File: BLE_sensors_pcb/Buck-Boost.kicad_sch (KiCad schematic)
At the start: 6 parts, among them U3 TPS63031DSK

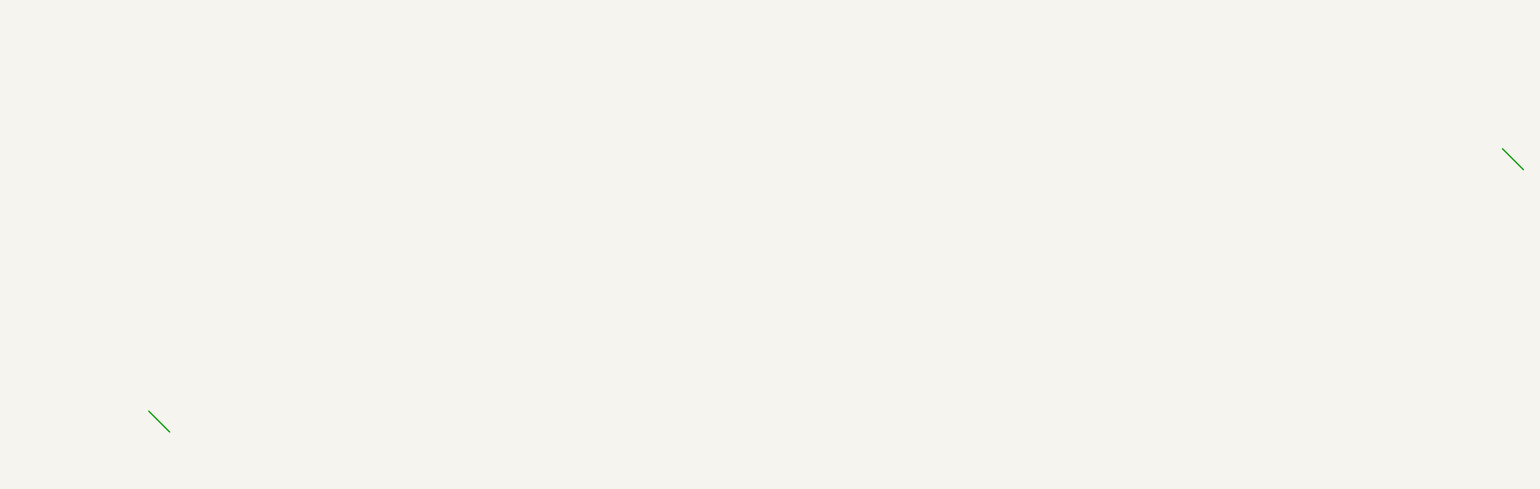
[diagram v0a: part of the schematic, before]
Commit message: save
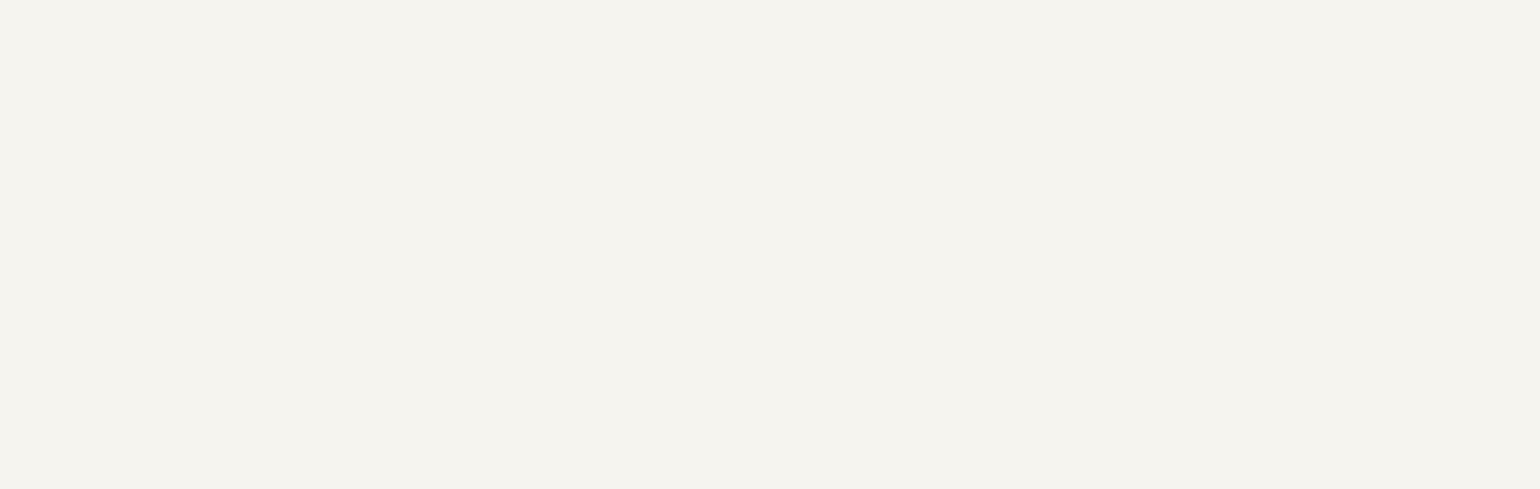
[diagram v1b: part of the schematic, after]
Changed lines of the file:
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@@
 		(color 0 0 0 0)
-	)
-	(bus_entry
-		(at 224.79 116.84)
-		(size 2.54 2.54)
-		(stroke
-			(width 0)
-			(type default)
-		)
-	)
-	(bus_entry
-		(at 388.62 85.09)
-		(size 2.54 2.54)
-		(stroke
-			(width 0)
-			(type default)
-		)
 	)
 	(wire
